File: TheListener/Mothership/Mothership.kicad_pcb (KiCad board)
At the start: 2 copper layers, 88.8 x 115.5 mm, 81 parts, among them J1 RJ45, J2 RJ45, J3 RJ45, J4 RJ45, J5 RJ45, J6 RJ45, J7 RJ45, J8 RJ45, J9 Conn_01x02_Female, U1 SP3491, U10 AMS1117-3.3, U11 NID35-5, U12 Teensy3.5, U2 SP3491, U3 SP3491, U4 SP3491, U5 SP3491, U6 SP3491, U7 SP3491, U8 SP3491, U9 AMS1117-3.3

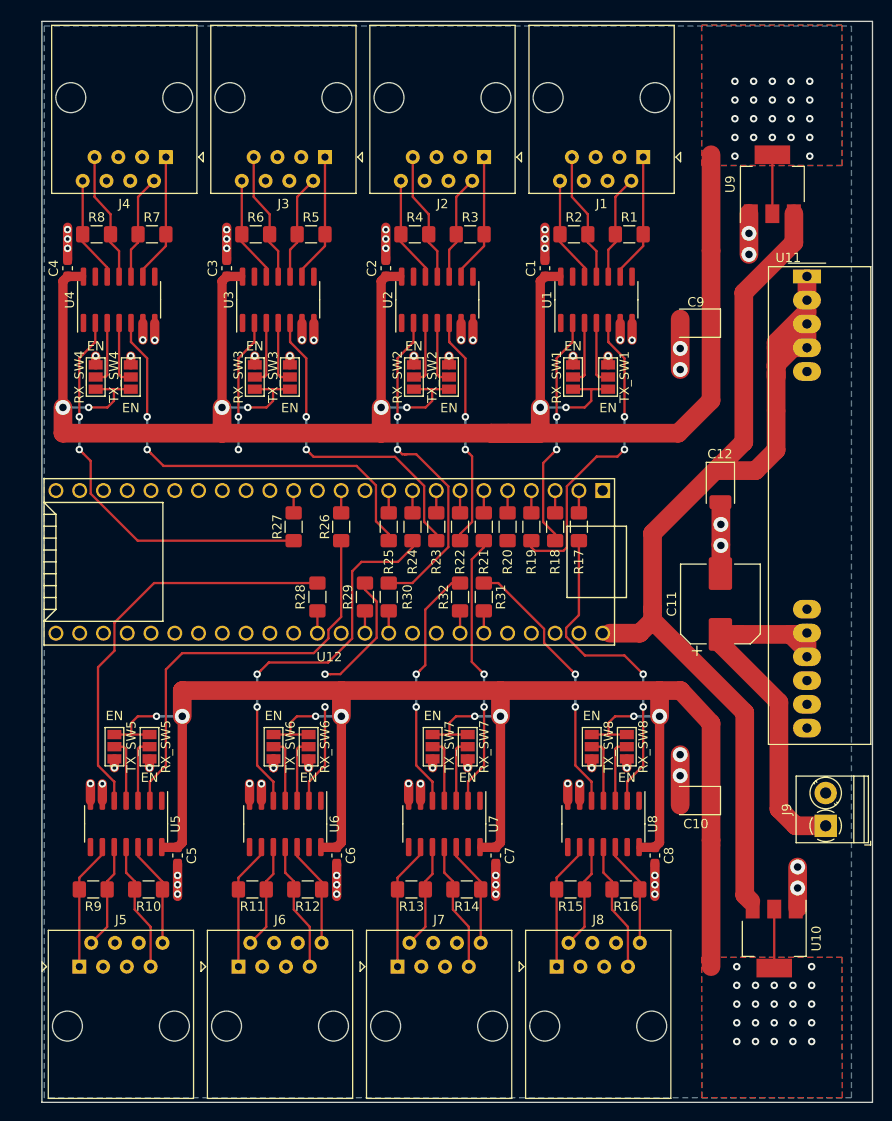
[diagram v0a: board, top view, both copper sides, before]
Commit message: wip
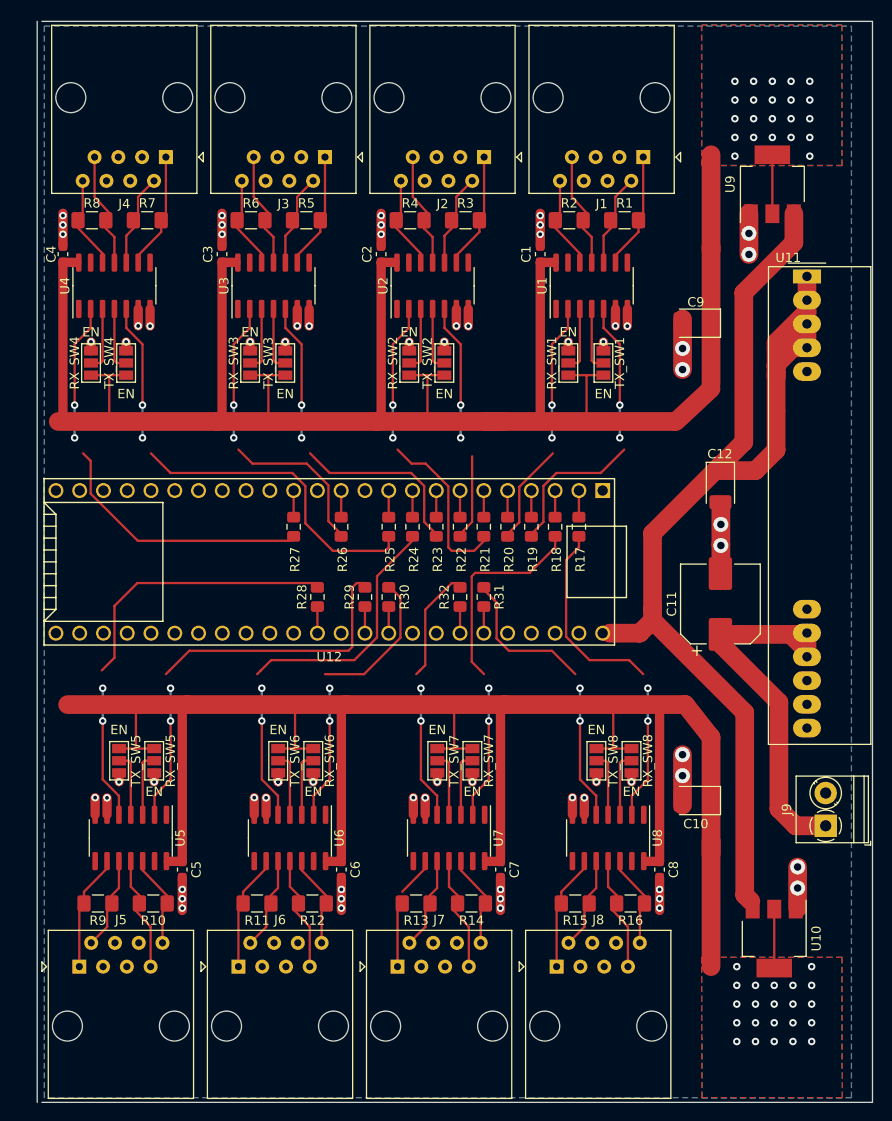
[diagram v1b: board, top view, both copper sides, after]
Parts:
- R17, R18, R19, R20, R21, R22, R23, R24, R25, R26, R27, R28, R29, R30, R31, R32: footprint Resistor_SMD:R_1206_3216Metric_Pad1.42x1.75mm_HandSolder -> Resistor_SMD:R_0805_2012Metric_Pad1.15x1.40mm_HandSolder
- moved C1 1.58 mm to (98.5, 46.4)
- moved C2 1.58 mm to (81.5, 46.4)
- moved C3 1.58 mm to (64.5, 46.4)
- moved C4 1.58 mm to (47.5, 46.4)
- moved C5 1.58 mm to (60.2, 112.1)
- moved C6 1.58 mm to (77.2, 112.1)
- moved C7 1.58 mm to (94.2, 112.1)
- moved C8 1.58 mm to (111.2, 112.1)
- moved R1 1.58 mm to (107.5, 42.8)
- moved R10 1.58 mm to (57.2, 115.8)
- moved R11 1.58 mm to (68.2, 115.8)
- moved R12 1.58 mm to (74.2, 115.8)
- moved R13 1.58 mm to (85.2, 115.8)
- moved R14 1.58 mm to (91.2, 115.8)
- moved R15 1.58 mm to (102.2, 115.8)
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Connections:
- R18 pad 2: R_1 -> R_7
- R20 pad 2: R_3 -> R_1
- R21 pad 2: R_7 -> R_2
- R26 pad 2: R_5 -> R_3
- R29 pad 2: R_6 -> R_5
- R30 pad 2: R_2 -> R_6
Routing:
- net VCC1: track 232.2 -> 211.8 mm, vias 30 -> 22
- net R_3: track 14.3 -> 31.9 mm
- net R_7: track 29.6 -> 36.2 mm
- net R_6: track 24.3 -> 30.3 mm
- net R_2: track 36.0 -> 32.3 mm
- net VCC2: track 211.7 -> 208.9 mm, vias 30 -> 22
- net Net-(J7-Pad1): track 13.8 -> 11.0 mm
- net T_1: track 33.4 -> 30.9 mm
- net Net-(J8-Pad7): track 13.8 -> 11.7 mm
- net Net-(J7-Pad7): track 13.8 -> 11.7 mm
- net Net-(J6-Pad7): track 13.8 -> 11.7 mm
- net Net-(J5-Pad7): track 13.8 -> 11.7 mm
- net Net-(J4-Pad7): track 13.8 -> 11.7 mm
- net Net-(J3-Pad7): track 13.8 -> 11.7 mm
- net Net-(J2-Pad7): track 13.8 -> 11.7 mm
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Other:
- board size 88.8 x 115.5 mm -> 89.2 x 115.5 mm

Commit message: wip
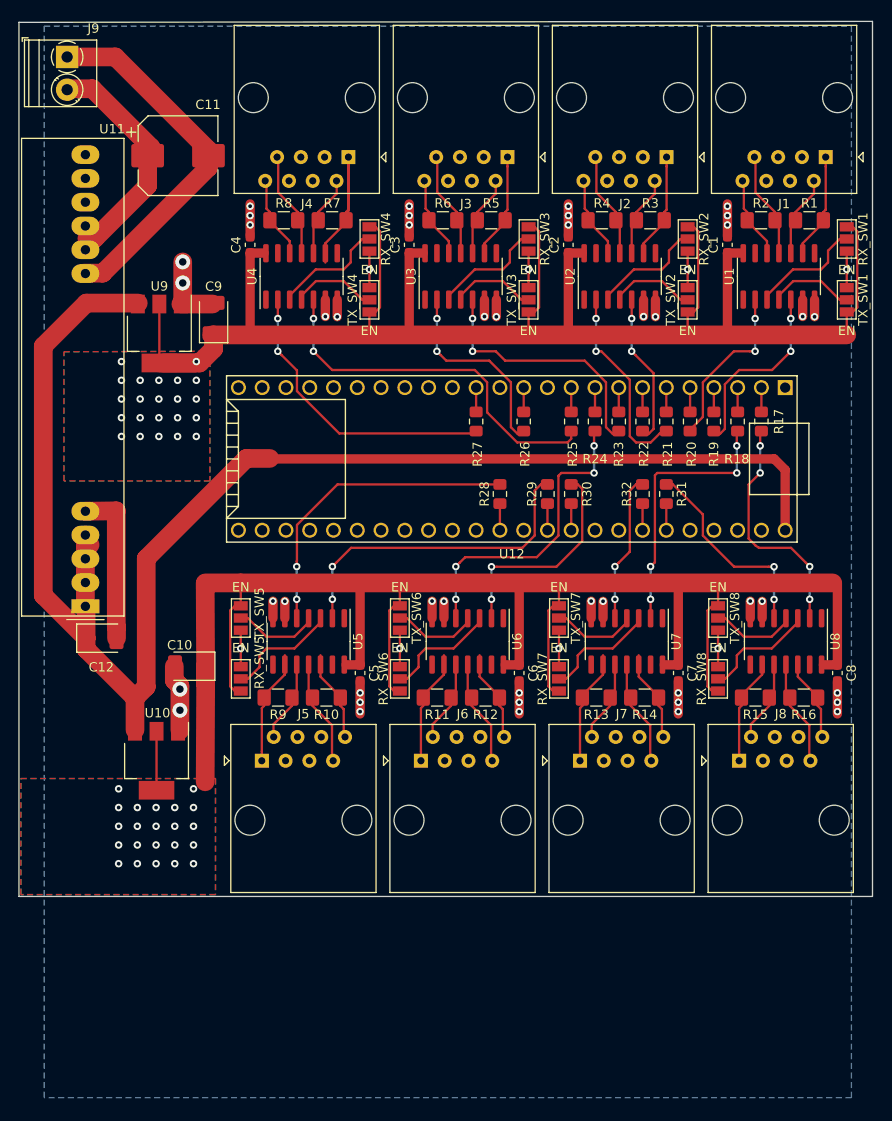
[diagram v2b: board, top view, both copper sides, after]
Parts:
- moved J9 115.4 mm to (48.0, 25.3), turned to 270 degrees
- moved U11 84.8 mm to (49.9, 84.0), turned to 180 degrees
- moved C11 75.2 mm to (59.8, 35.9), turned to 0 degrees
- moved U10 68.7 mm to (57.5, 100.5)
- moved C12 68.1 mm to (51.6, 87.4), turned to 0 degrees
- moved U9 67.4 mm to (57.8, 54.9), turned to 270 degrees
- moved C10 55.9 mm to (61.1, 90.4)
- moved C9 51.5 mm to (63.6, 53.2), turned to 90 degrees
- moved RX_SW1 32.6 mm to (131.2, 44.8), turned to 90 degrees
- moved RX_SW2 32.6 mm to (114.2, 44.8), turned to 90 degrees
- moved RX_SW3 32.6 mm to (97.2, 44.8), turned to 90 degrees
- moved RX_SW4 32.6 mm to (80.2, 44.8), turned to 90 degrees
- moved J5 29.4 mm to (68.8, 100.5)
- moved J6 29.4 mm to (85.8, 100.5)
- moved J7 29.4 mm to (102.8, 100.5)
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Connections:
- J9 pad 1: +24V -> GND
- J9 pad 2: GND -> +24V
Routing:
- net GND: track 99.2 -> 159.8 mm, vias 67 -> 52
- net +5V: track 128.5 -> 163.6 mm
- net VCC1: track 211.8 -> 179.3 mm
- net VCC2: track 208.9 -> 190.2 mm
- net +24V: track 41.5 -> 24.2 mm
- net R_2: track 32.3 -> 21.0 mm
- net T_5: track 44.4 -> 33.5 mm
- net T_1: track 30.9 -> 20.2 mm
- net R_4: track 42.4 -> 31.6 mm
- net R_3: track 31.9 -> 21.2 mm
- net T_7: track 26.4 -> 15.9 mm
- net R_8: track 35.2 -> 25.0 mm, vias 2 -> 4
- net R_5: track 44.0 -> 34.9 mm
- net T_6: track 40.6 -> 32.2 mm, vias 2 -> 4
- net T_8: track 30.7 -> 22.7 mm
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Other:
- board size 89.2 x 115.5 mm -> 91.2 x 93.5 mm
